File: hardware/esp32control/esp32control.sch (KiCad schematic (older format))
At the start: 62 parts, among them J1 Conn_02x10_Odd_Even, Q5 BSS138, Q6 BSS138, Q7 MMBT3904, Q8 MMBT3904, SW1 Boot, SW2 Reset, U1 ESP32-WROOM, U10 LTV-354T, U11 HUT4, U12 LM1117-3.3, U13 RV-8523-C3, U4 LM2675M-5, U5 LTV-354T, U8 LTV-354T, U9 LTV-354T

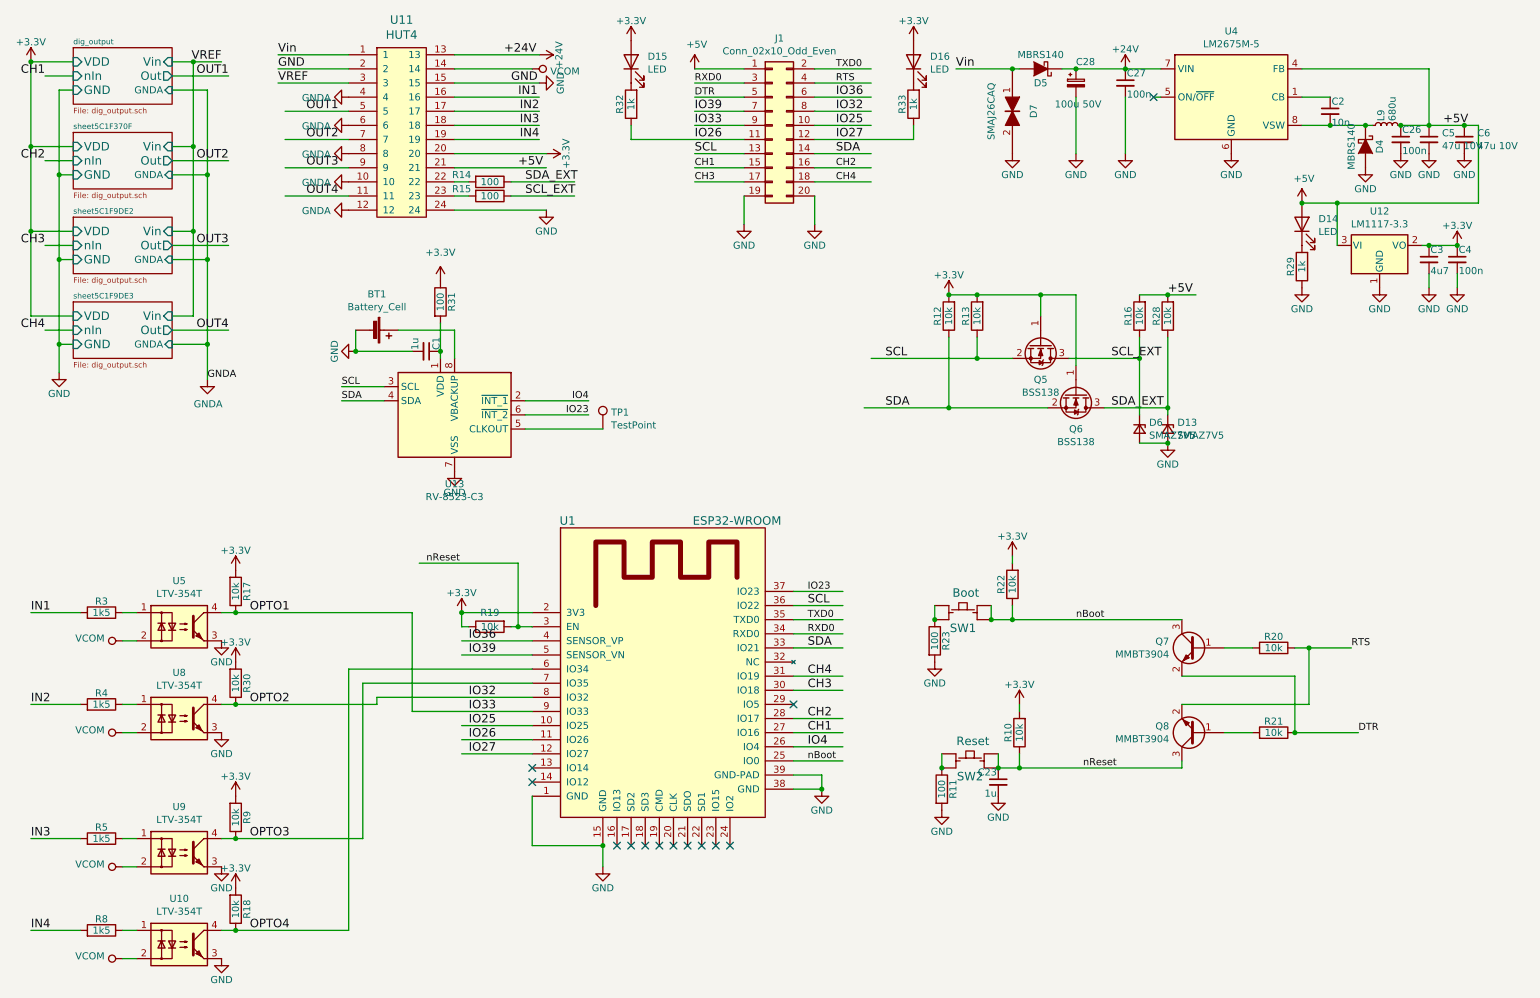
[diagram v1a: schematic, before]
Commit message: kicad6 update
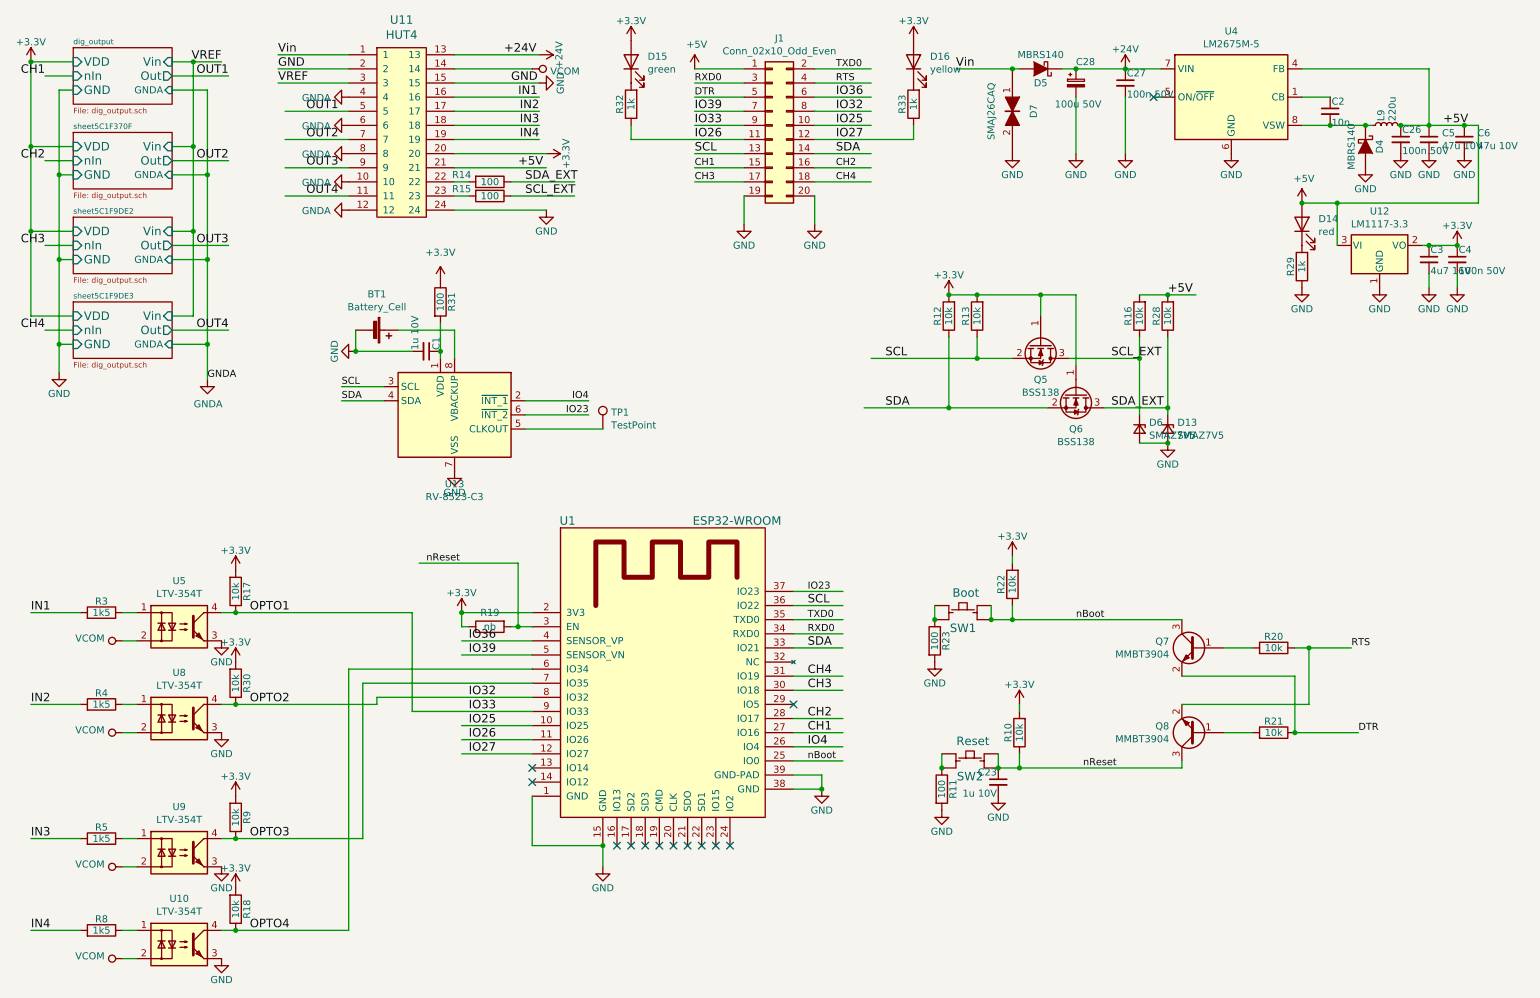
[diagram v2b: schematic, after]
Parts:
- C1, C23: value 1u -> 1u 10V; Mouser (none) -> 963-LMK107B7105KA-T
- C26, C27, C4: value 100n -> 100n 50V; Mouser (none) -> 80-C0603C104M5R
- C3: value 4u7 -> 4u7 16V; Mouser (none) -> 710-885012107013
- C5, C6: Mouser (none) -> 963-LMK316BC6476ML-T
- D14: value LED -> red; Mouser (none) -> 710-150060RS75000
- D15: value LED -> green; Mouser (none) -> 710-150060GS75000
- D16: value LED -> yellow; Mouser (none) -> 710-150060YS75000
- L9: value 680u -> 220u; Mouser (none) -> 710-74477728; Wuerth 74477728 -> (none)
- R19: value 10k -> nb
- U1: Mouser (none) -> 356-ESP32WRM32UE28UH
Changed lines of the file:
@@
 P 7750 6050
 F 0 "C23" H 7760 6120 50  0000 L CNN
-F 1 "1u" H 7760 5970 50  0000 L CNN
+F 1 "1u 10V" H 7760 5970 50  0000 L CNN
 F 2 "Capacitor_SMD:C_0603_1608Metric" H 7750 6050 60  0001 C CNN
 F 3 "" H 7750 6050 60  0000 C CNN
+F 4 " 963-LMK107B7105KA-T " H 7750 6050 50  0001 C CNN "Mouser"
 	1    7750 6050
 	-1   0    0    -1
@@
 P 10500 1400
 F 0 "L9" H 10530 1440 50  0000 L CNN
-F 1 "680u" H 10530 1360 50  0000 L CNN
+F 1 "220u" H 10530 1360 50  0000 L CNN
 F 2 "Inductor_SMD:L_7.3x7.3_H4.5" H 10500 1400 60  0001 C CNN
 F 3 "" H 10500 1400 60  0000 C CNN
-F 4 "74477728" H 10500 1400 60  0001 C CNN "Wuerth"
+F 4 "" H 10500 1400 60  0001 C CNN "Wuerth"
+F 5 " 710-74477728 " H 10500 1400 50  0001 C CNN "Mouser"
 	1    10500 1400
 	0    -1   -1   0
@@
 P 8650 1100
 F 0 "C27" H 8660 1170 50  0000 L CNN
-F 1 "100n" H 8660 1020 50  0000 L CNN
+F 1 "100n 50V" H 8660 1020 50  0000 L CNN
 F 2 "Capacitor_SMD:C_0603_1608Metric" H 8650 1100 60  0001 C CNN
 F 3 "" H 8650 1100 60  0000 C CNN
+F 4 " 80-C0603C104M5R " H 8650 1100 50  0001 C CNN "Mouser"
 	1    8650 1100
 	1    0    0    -1
@@
 P 10600 1500
 F 0 "C26" H 10610 1570 50  0000 L CNN
-F 1 "100n" H 10610 1420 50  0000 L CNN
+F 1 "100n 50V" H 10610 1420 50  0000 L CNN
 F 2 "Capacitor_SMD:C_0603_1608Metric" H 10600 1500 60  0001 C CNN
 F 3 "" H 10600 1500 60  0000 C CNN
+F 4 " 80-C0603C104M5R " H 10600 1500 50  0001 C CNN "Mouser"
 	1    10600 1500
 	1    0    0    -1
@@
 F 2 "ESP32-footprints-Lib:ESP32-WROOM" H 5750 6800 60  0001 C CNN
 F 3 "" H 4950 5900 60  0001 C CNN
+F 4 " 356-ESP32WRM32UE28UH " H 5400 5450 50  0001 C CNN "Mouser"
 	1    5400 5450
 	1    0    0    -1
@@
 P 4150 4950
 F 0 "R19" V 4050 4950 50  0000 C CNN
-F 1 "10k" V 4150 4950 50  0000 C CNN
+F 1 "nb" V 4150 4950 50  0000 C CNN
 F 2 "Resistor_SMD:R_0603_1608Metric" V 4080 4950 30  0001 C CNN
 F 3 "" H 4150 4950 30  0000 C CNN
@@
 P 11000 2350
 F 0 "C4" H 11010 2420 50  0000 L CNN
-F 1 "100n" H 11010 2270 50  0000 L CNN
+F 1 "100n 50V" H 11010 2270 50  0000 L CNN
 F 2 "Capacitor_SMD:C_0603_1608Metric" H 11000 2350 60  0001 C CNN
 F 3 "" H 11000 2350 60  0000 C CNN
+F 4 " 80-C0603C104M5R " H 11000 2350 50  0001 C CNN "Mouser"
 	1    11000 2350
 	1    0    0    -1
@@
 P 10800 2350
 F 0 "C3" H 10810 2420 50  0000 L CNN
-F 1 "4u7" H 10810 2270 50  0000 L CNN
+F 1 "4u7 16V" H 10810 2270 50  0000 L CNN
 F 2 "Capacitor_SMD:C_0805_2012Metric_Pad1.15x1.40mm_HandSolder" H 10800 2350 60  0001 C CNN
 F 3 "" H 10800 2350 60  0000 C CNN
+F 4 " 710-885012107013 " H 10800 2350 50  0001 C CNN "Mouser"
 	1    10800 2350
 	1    0    0    -1
@@
 P 9900 2100
 F 0 "D14" V 9938 1983 50  0000 R CNN
-F 1 "LED" V 9847 1983 50  0000 R CNN
+F 1 "red" V 9847 1983 50  0000 R CNN
 F 2 "LED_SMD:LED_0603_1608Metric_Pad1.05x0.95mm_HandSolder" H 9900 2100 50  0001 C CNN
 F 3 "~" H 9900 2100 50  0001 C CNN
+F 4 " 710-150060RS75000 " H 9900 2100 50  0001 C CNN "Mouser"
 	1    9900 2100
 	0    -1   -1   0
@@
 P 3700 3000
 F 0 "C1" H 3710 3070 50  0000 L CNN
-F 1 "1u" H 3710 2920 50  0000 L CNN
+F 1 "1u 10V" H 3710 2920 50  0000 L CNN
 F 2 "Capacitor_SMD:C_0603_1608Metric" H 3700 3000 60  0001 C CNN
 F 3 "" H 3700 3000 60  0000 C CNN
+F 4 " 963-LMK107B7105KA-T " H 3700 3000 50  0001 C CNN "Mouser"
 	1    3700 3000
 	0    1    -1   0
@@
 P 5150 950
 F 0 "D15" V 5188 833 50  0000 R CNN
-F 1 "LED" V 5097 833 50  0000 R CNN
+F 1 "green" V 5097 833 50  0000 R CNN
 F 2 "LED_SMD:LED_0603_1608Metric_Pad1.05x0.95mm_HandSolder" H 5150 950 50  0001 C CNN
 F 3 "~" H 5150 950 50  0001 C CNN
+F 4 " 710-150060GS75000 " H 5150 950 50  0001 C CNN "Mouser"
 	1    5150 950
 	0    -1   -1   0
@@
 P 7150 950
 F 0 "D16" V 7188 833 50  0000 R CNN
-F 1 "LED" V 7097 833 50  0000 R CNN
+F 1 "yellow" V 7097 833 50  0000 R CNN
 F 2 "LED_SMD:LED_0603_1608Metric_Pad1.05x0.95mm_HandSolder" H 7150 950 50  0001 C CNN
 F 3 "~" H 7150 950 50  0001 C CNN
+F 4 " 710-150060YS75000 " H 7150 950 50  0001 C CNN "Mouser"
 	1    7150 950
 	0    -1   -1   0
@@
 F 2 "Capacitor_SMD:C_1206_3216Metric" H 10800 1500 50  0001 C CNN
 F 3 "~" H 10800 1500 50  0001 C CNN
+F 4 " 963-LMK316BC6476ML-T " H 10800 1500 50  0001 C CNN "Mouser"
 	1    10800 1500
 	1    0    0    -1
@@
 F 2 "Capacitor_SMD:C_1206_3216Metric" H 11050 1500 50  0001 C CNN
 F 3 "~" H 11050 1500 50  0001 C CNN
+F 4 " 963-LMK316BC6476ML-T " H 11050 1500 50  0001 C CNN "Mouser"
 	1    11050 1500
 	1    0    0    -1
